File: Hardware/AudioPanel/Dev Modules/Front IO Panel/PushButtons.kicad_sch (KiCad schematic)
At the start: 80 parts, among them CN501 4x 10nF, CN502 4x 10nF, CN503 4x 10nF, U501 74HC14, U502 74HC14, U503 74HC14, U504 74HC14, U505 74HC14, U506 74HC14, U507 MCP23017_ML, U508 74HC14, U509 74HC14, U510 74HC14, U511 74HC14, U512 74HC14, U513 74HC14

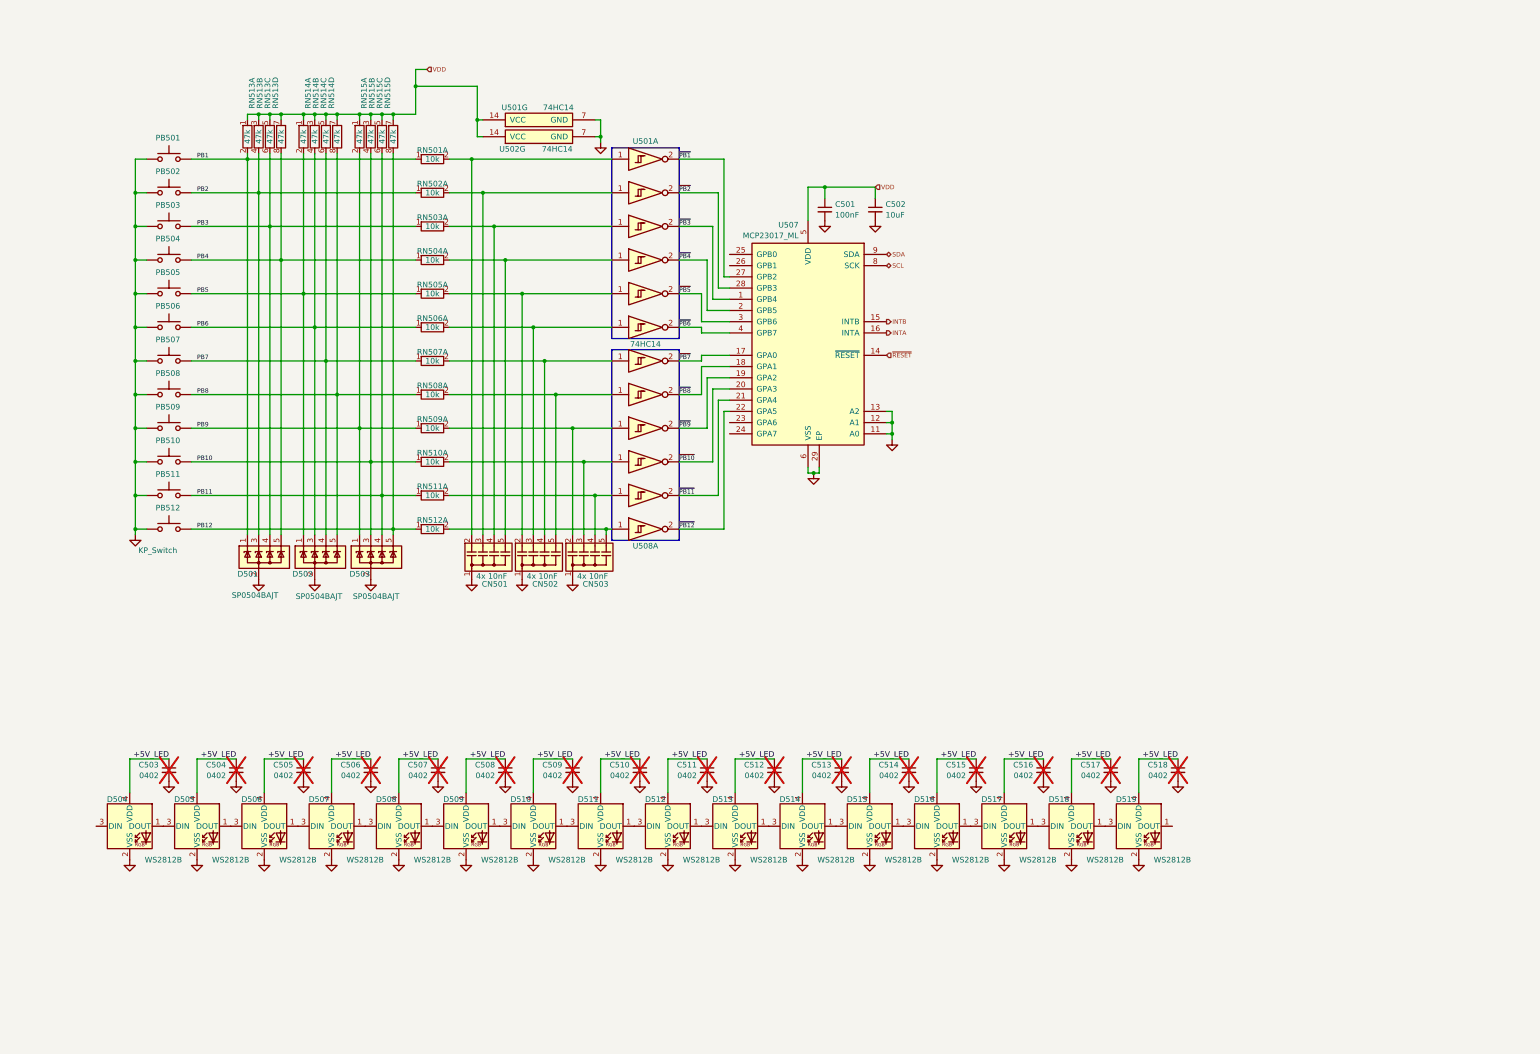
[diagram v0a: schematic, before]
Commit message: IO Panel Progress
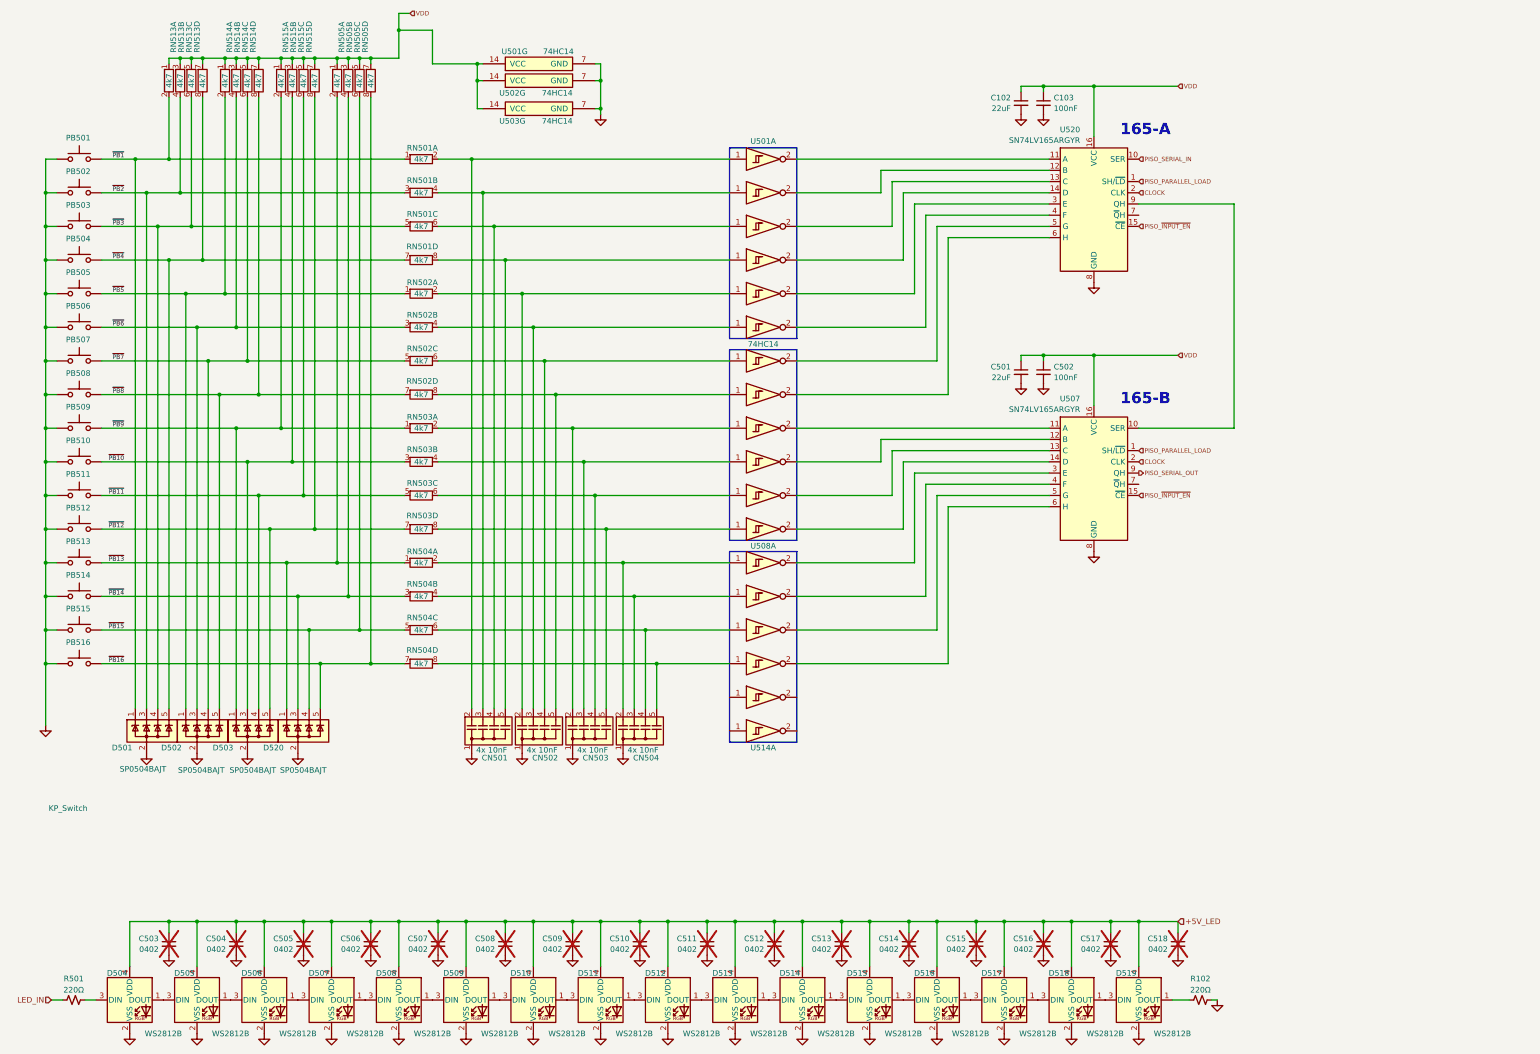
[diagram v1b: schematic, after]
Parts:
- removed RN501, RN502, RN503, RN504, RN505, RN506, RN507, RN508, RN509, RN510, RN511, RN512: 10k, Resistor_THT:R_Array_SIP5, symbol Device:R_Network04_Split
- removed U507: MCP23017_ML, Package_DFN_QFN:QFN-28-1EP_6x6mm_P0.65mm_EP4.25x4.25mm, symbol Interface_Expansion:MCP23017_ML
- added C102: 22uF, Libraries:Worthington_C_0603, symbol Device:C_Small
- added C103: 100nF, Libraries:Worthington_C_0402, symbol Device:C_Small
- added CN504: 4x 10nF, symbol Device:C_Network04
- added D520: SP0504BAJT, Package_TO_SOT_SMD:SOT-353_SC-70-5, symbol Power_Protection:SP0504BAJT
- added PB513, PB514, PB515, PB516: KP_Switch, symbol Switch:SW_Push
- added R102, R501: 220Ω, Libraries:Worthington_R_0402, symbol Device:R_Small_US
- added RN501, RN502, RN503, RN504, RN505: 4k7, Resistor_SMD:R_Array_Convex_4x1206, symbol Library_MicSwitcher:R_Network04_Split
- added unit 7 of U503
- added U507, U520: SN74LV165ARGYR, Libraries:RGY16_2P55X2P05, symbol Libraries:74HC165
- added U514, U515, U516, U517, U518, U519: 74HC14, symbol AudioPanelLibrary:74HC14
- C501: value 100nF -> 22uF; footprint (none) -> Libraries:Worthington_C_0603
- C502: value 10uF -> 100nF; footprint (none) -> Libraries:Worthington_C_0402
- RN513, RN514, RN515: value 47k -> 4k7
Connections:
- net PB1 is gone; now on net ~{PB1}: D501.1 (K), PB501.2, RN513.2
- net PB10 is gone; now on net ~{PB10}: D503.3 (K), PB510.2, RN515.4
- net PB11 is gone; now on net ~{PB11}: D503.4 (K), PB511.2, RN515.6
- net PB12 is gone; now on net ~{PB12}: D503.5 (K), PB512.2, RN515.8
- net PB2 is gone; now on net ~{PB2}: D501.3 (K), PB502.2, RN513.4
- net PB3 is gone; now on net ~{PB3}: D501.4 (K), PB503.2, RN513.6
- net PB4 is gone; now on net ~{PB4}: D501.5 (K), PB504.2, RN513.8
- net PB5 is gone; now on net ~{PB5}: D502.1 (K), PB505.2, RN514.2
- net PB6 is gone; now on net ~{PB6}: D502.3 (K), PB506.2, RN514.4
- net PB7 is gone; now on net ~{PB7}: D502.4 (K), PB507.2, RN514.6
- net PB8 is gone; now on net ~{PB8}: D502.5 (K), PB508.2, RN514.8
- net PB9 is gone; now on net ~{PB9}: D503.1 (K), PB509.2, RN515.2
- net GND: now also C102.2, C103.2, CN504.1 (common), D520.2 (A), PB513.1, PB514.1, PB515.1, PB516.1, R102.2, U503.7 (GND), U507.8 (GND), U520.8 (GND)
- net VDD: now also C102.1, C103.1, RN505.1, RN505.3, RN505.5, RN505.7, U503.14 (VCC), U507.16 (VCC), U520.16 (VCC)
- net ~{PB10}: now also RN503.3; no longer U511.2
- net ~{PB11}: now also RN503.5; no longer U512.2
- net ~{PB12}: now also RN503.7; no longer U513.2
- net ~{PB1}: now also RN501.1; no longer U501.2
- net ~{PB2}: now also RN501.3; no longer U502.2
- net ~{PB3}: now also RN501.5; no longer U503.2
- net ~{PB4}: now also RN501.7; no longer U504.2
- net ~{PB5}: now also RN502.1; no longer U505.2
- net ~{PB6}: now also RN502.3; no longer U506.2
- net ~{PB7}: now also RN502.5; no longer U508.2
- net ~{PB8}: now also RN502.7; no longer U509.2
- net ~{PB9}: now also RN503.1; no longer U510.2
- net at CN502.2 (C1), U505.1: now also RN502.2
- net at CN503.2 (C1), U510.1: now also RN503.2
- net at CN503.3 (C2), U511.1: now also RN503.4
- net at CN503.4 (C3), U512.1: now also RN503.6
- net at CN503.5 (C4), U513.1: now also RN503.8
- net at D519.1 (DOUT): now also R102.1
- net at CN501.5 (C4), U504.1: now also RN501.8
- net at CN501.4 (C3), U503.1: now also RN501.6
- net at CN501.2 (C1), U501.1: now also RN501.2
- net at CN502.5 (C4), U509.1: now also RN502.8
- net at CN501.3 (C2), U502.1: now also RN501.4
- net at CN502.3 (C2), U506.1: now also RN502.4
- net at D504.3 (DIN): now also R501.2
- net at CN502.4 (C3), U508.1: now also RN502.6
- new net: CN504.2 (C1), RN504.2, U514.1
- new net: U507.3 (E), U514.2
- new net: U505.2, U520.3 (E)
- new net: CN504.3 (C2), RN504.4, U515.1
- new net: U504.2, U520.14 (D)
- new net: CN504.4 (C3), RN504.6, U516.1
- new net: U507.5 (G), U516.2
- new net: U503.2, U520.13 (C)
- new net: U501.2, U520.11 (A)
- new net: U502.2, U520.12 (B)
- new net: U506.2, U520.4 (F)
- new net: U508.2, U520.5 (G)
- new net: U509.2, U520.6 (H)
- new net: U507.10 (SER), U520.9 (QH)
- new net: U507.14 (D), U513.2
- new net: U507.11 (A), U510.2
- new net: U507.4 (F), U515.2
- new net: CN504.5 (C4), RN504.8, U517.1
- new net: U507.13 (C), U512.2
- new net: U507.6 (H), U517.2
- new net: U507.12 (B), U511.2
- new net CLOCK: U507.2 (CLK), U520.2 (CLK)
- new net LED_IN: R501.1
- new net PISO_PARALLEL_LOAD: U507.1 (SH/~{LD}), U520.1 (SH/~{LD})
- new net PISO_SERIAL_IN: U520.10 (SER)
- new net PISO_SERIAL_OUT: U507.9 (QH)
- new net PISO_~{INPUT_EN}: U507.15 (~{CE}), U520.15 (~{CE})
- new net ~{PB13}: D520.1 (K), PB513.2, RN504.1, RN505.2
- new net ~{PB14}: D520.3 (K), PB514.2, RN504.3, RN505.4
- new net ~{PB15}: D520.4 (K), PB515.2, RN504.5, RN505.6
- new net ~{PB16}: D520.5 (K), PB516.2, RN504.7, RN505.8
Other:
- note added: "165-A"
- note added: "165-B"
- moved on the sheet: C503, C504, C505, C506, C507, C508, C509, C510, C511, C512, C513, C514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

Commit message: Work on front control panel
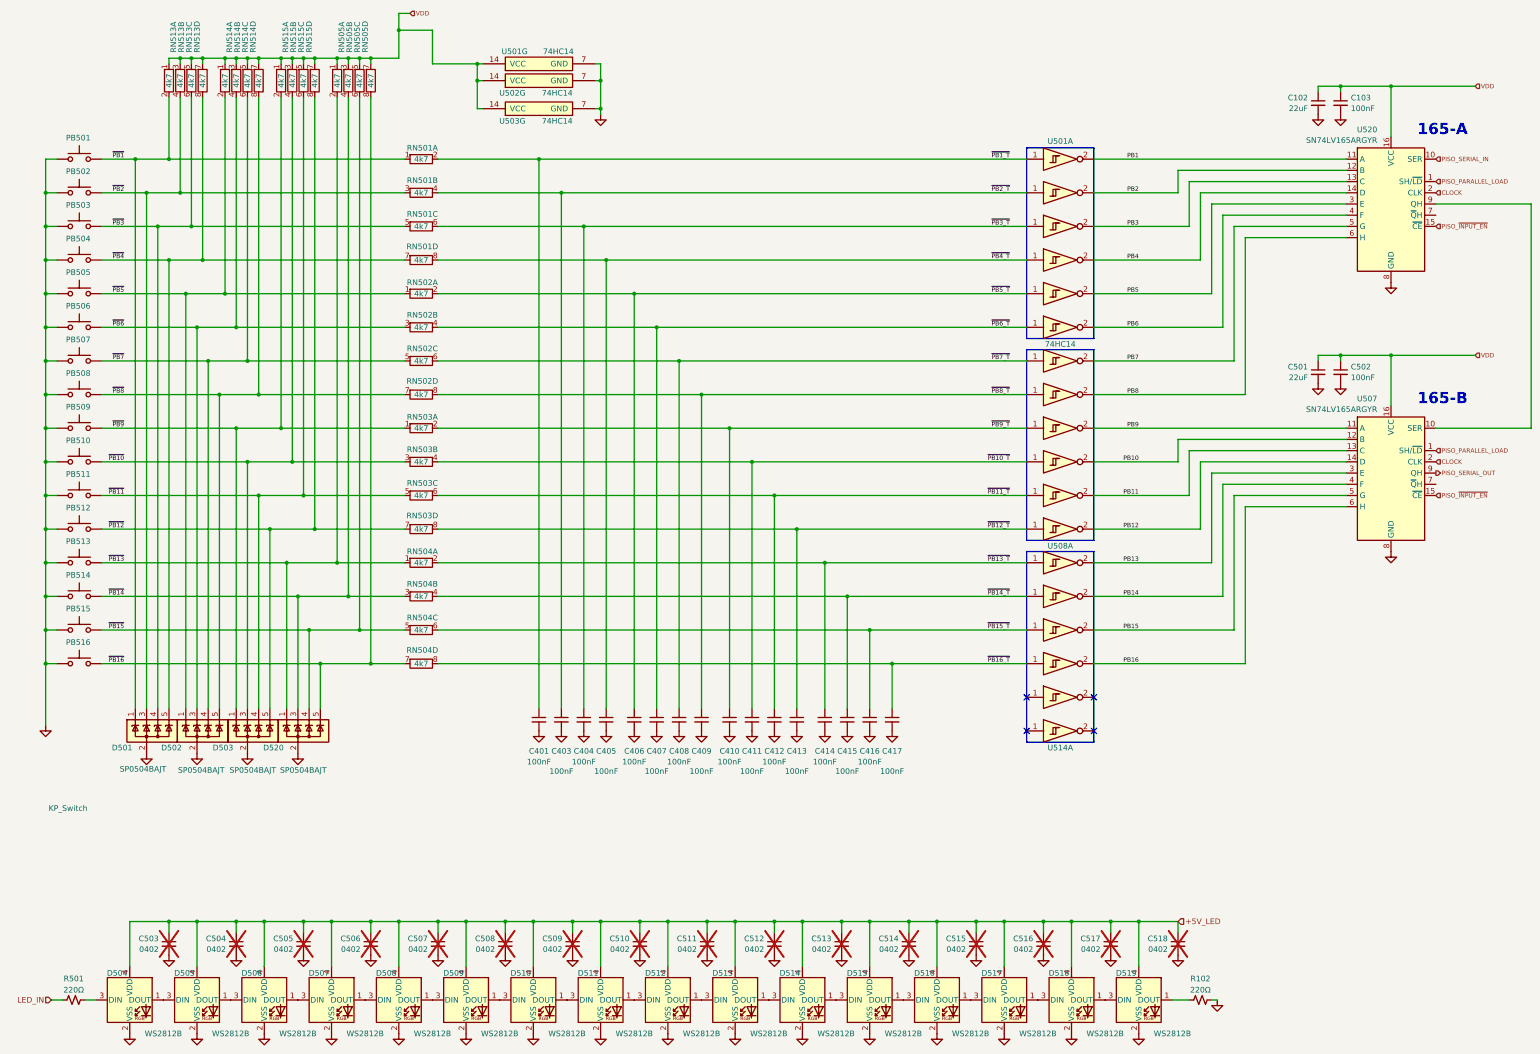
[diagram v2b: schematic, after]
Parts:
- removed CN501, CN502, CN503, CN504: 4x 10nF, symbol Device:C_Network04
- added C401, C403, C404, C405, C406, C407, C408, C409, C410, C411, C412, C413, C414, C415, C416, C417: 100nF, Libraries:Worthington_C_0402, symbol Device:C_Small
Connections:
- net GND: now also C401.2, C403.2, C404.2, C405.2, C406.2, C407.2, C408.2, C409.2, C410.2, C411.2, C412.2, C413.2, C414.2, C415.2, C416.2, C417.2
- net ~{PB13_T}: now reaches RN504.2, U514.1
- net ~{PB13_T}: now also C414.1
- net PB13: now reaches U507.3 (E), U514.2
- net ~{PB5_T}: now reaches RN502.2, U505.1
- net ~{PB5_T}: now also C406.1
- net PB5: now reaches U505.2, U520.3 (E)
- net ~{PB9_T}: now reaches RN503.2, U510.1
- net ~{PB9_T}: now also C410.1
- net ~{PB10_T}: now reaches RN503.4, U511.1
- net ~{PB10_T}: now also C411.1
- net ~{PB11_T}: now reaches RN503.6, U512.1
- net ~{PB11_T}: now also C412.1
- net ~{PB12_T}: now reaches RN503.8, U513.1
- net ~{PB12_T}: now also C413.1
- net ~{PB14_T}: now reaches RN504.4, U515.1
- net ~{PB14_T}: now also C415.1
- net ~{PB6_T}: now reaches RN502.4, U506.1
- net ~{PB6_T}: now also C407.1
- net ~{PB4_T}: now reaches RN501.8, U504.1
- net ~{PB4_T}: now also C405.1
- net PB4: now reaches U504.2, U520.14 (D)
- net ~{PB15_T}: now reaches RN504.6, U516.1
- net ~{PB15_T}: now also C416.1
- net PB15: now reaches U507.5 (G), U516.2
- net ~{PB3_T}: now reaches RN501.6, U503.1
- net ~{PB3_T}: now also C404.1
- net PB3: now reaches U503.2, U520.13 (C)
- net PB1: now reaches U501.2, U520.11 (A)
- net PB2: now reaches U502.2, U520.12 (B)
- net PB6: now reaches U506.2, U520.4 (F)
- net PB7: now reaches U508.2, U520.5 (G)
- net PB8: now reaches U509.2, U520.6 (H)
- net PB12: now reaches U507.14 (D), U513.2
- net ~{PB1_T}: now reaches RN501.2, U501.1
- net ~{PB1_T}: now also C401.1
- net PB9: now reaches U507.11 (A), U510.2
- net ~{PB8_T}: now reaches RN502.8, U509.1
- net ~{PB8_T}: now also C409.1
- net PB14: now reaches U507.4 (F), U515.2
- net ~{PB16_T}: now reaches RN504.8, U517.1
- net ~{PB16_T}: now also C417.1
- net ~{PB2_T}: now reaches RN501.4, U502.1
- net ~{PB2_T}: now also C403.1
- net PB11: now reaches U507.13 (C), U512.2
- net PB16: now reaches U507.6 (H), U517.2
- net PB10: now reaches U507.12 (B), U511.2
- net ~{PB7_T}: now reaches RN502.6, U508.1
- net ~{PB7_T}: now also C408.1
- no-connect marks 0 -> 4
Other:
- moved on the sheet: C102, C103, C501, C502, U501A, U507, U508A, U514A, U520
